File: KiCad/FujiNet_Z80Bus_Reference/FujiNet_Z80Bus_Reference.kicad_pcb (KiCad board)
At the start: 2 copper layers, 180.3 x 119.4 mm, 77 parts, among them IC1 74244N, IC10 74595N, IC11 74595N, IC12 74165N, IC13 7432N, IC14 74165N, IC15 7408N, IC16 74165N, IC17 74165N, IC19 7432N, IC2 7404N, IC20 7408N, IC21 7432N, IC22 7432N, IC3 7474N, IC4 7432N, IC5 7408N, IC6 74590N, IC7 74590N, IC8 74595N, IC9 74595N, J2 DIAG-ESP_SPI, J3 DIAG-Z80_CONTROL, J4 DIAG-ESP_CONTROL, J5 DIAG-LOCAL_ADD_HIGH, J6 DIAG-LOCAL_ADD_LOW, J7 DIAG-LOCAL_DATA, J8 DIAG-HOST_SYSTEM_BUS, Q1 2N2222 (BC337), U1 FREENOVE_ESP32-WROVER-DEV

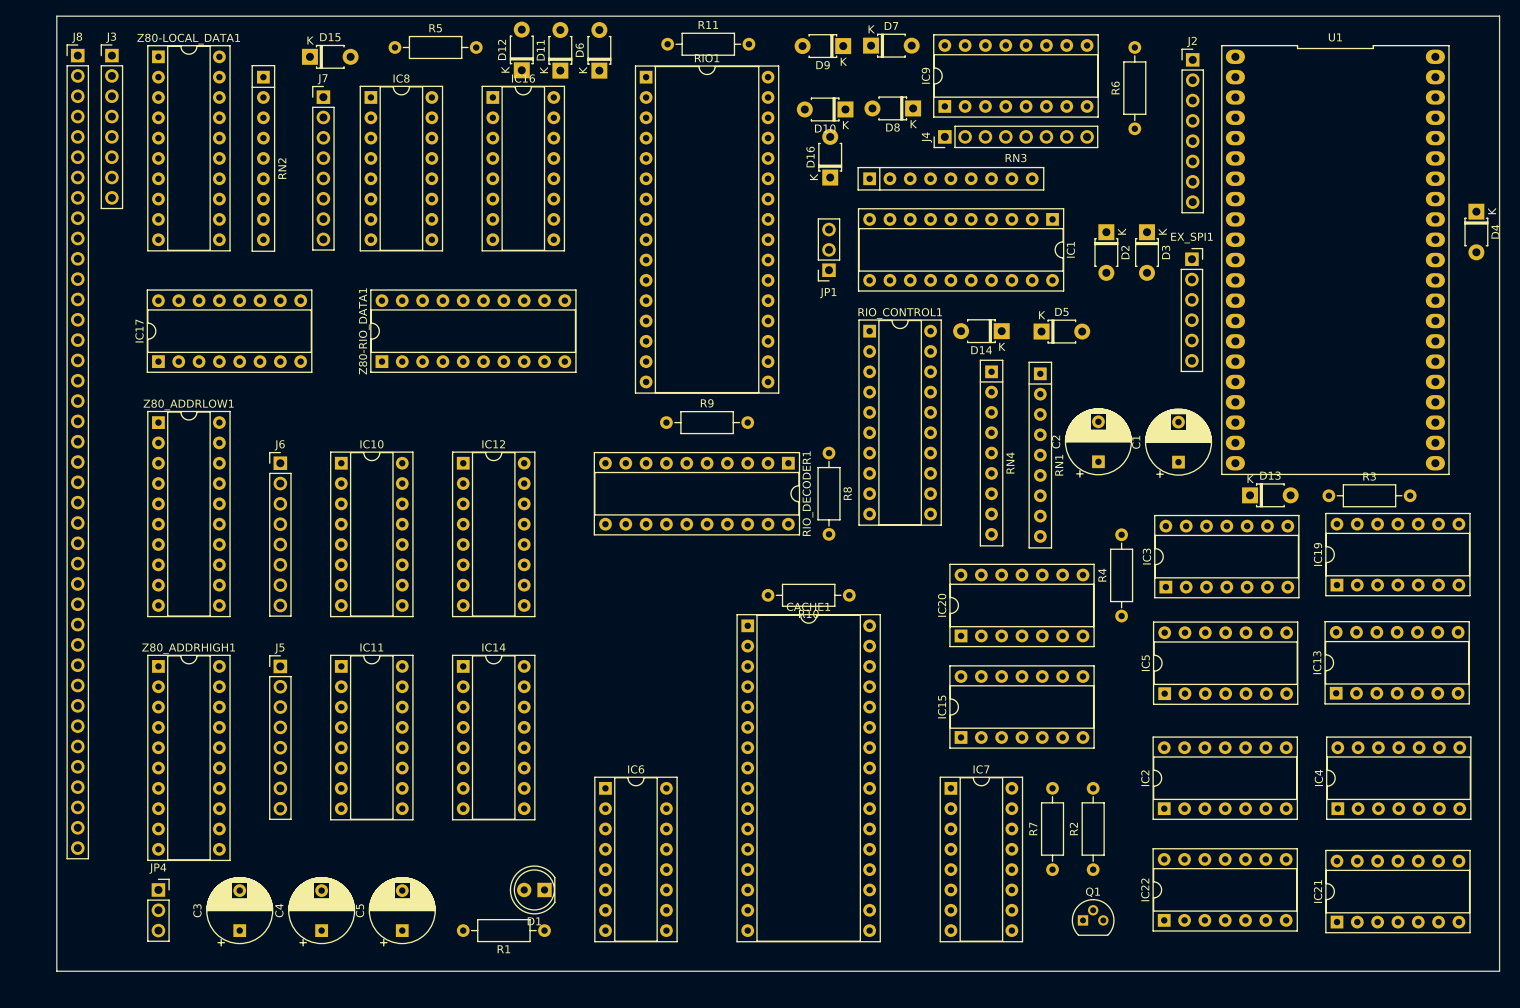
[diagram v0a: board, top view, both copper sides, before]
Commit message: Single PCB layout experiements
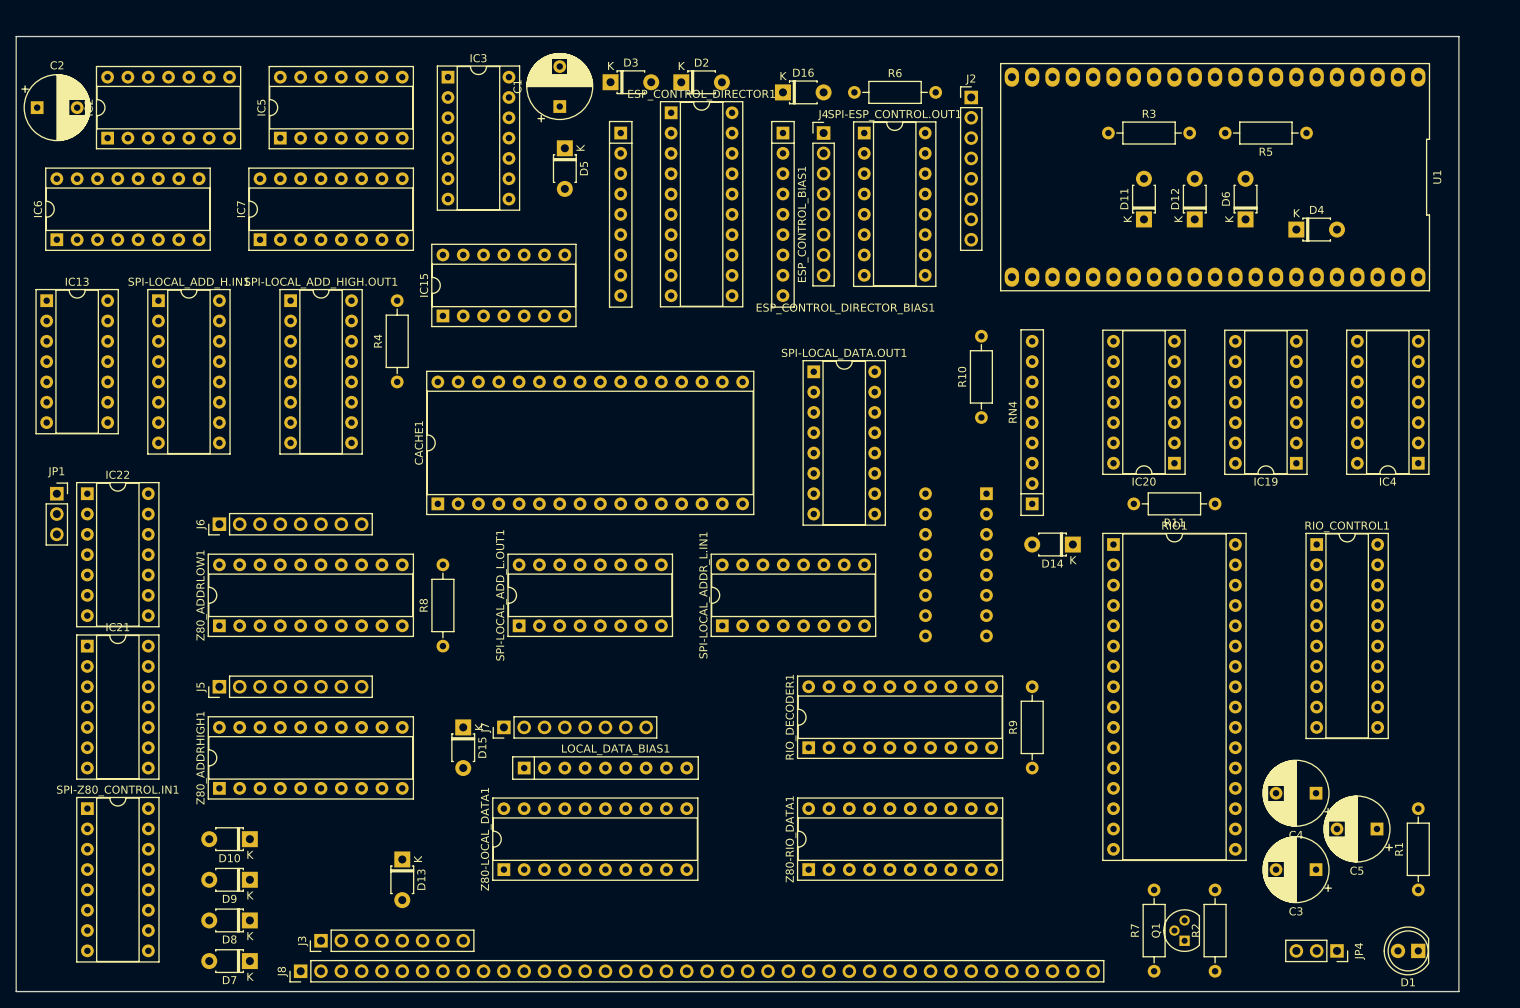
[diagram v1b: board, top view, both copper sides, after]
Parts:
- removed EX_SPI1: PINHD-1X6, Connector_PinSocket_2.54mm:PinSocket_1x06_P2.54mm_Vertical
- removed IC1: 74244N, Package_DIP:DIP-20_W7.62mm_Socket
- removed IC10, IC11, IC8, IC9: 74595N, Package_DIP:DIP-16_W7.62mm_Socket
- removed IC12, IC14, IC16, IC17: 74165N, Package_DIP:DIP-16_W7.62mm_Socket
- removed RN1, RN2, RN3: 4609M-101-103LF, Resistor_THT:R_Array_SIP9
- added ESP_CONTROL_BIAS1: 4609M-101-103LF, Resistor_THT:R_Array_SIP9, F.Cu at (133.9, 47.6)
- added ESP_CONTROL_DIRECTOR1: 74244N, Package_DIP:DIP-20_W7.62mm_Socket, F.Cu at (120.0, 45.1)
- added ESP_CONTROL_DIRECTOR_BIAS1: 4609M-101-103LF, Resistor_THT:R_Array_SIP9, F.Cu at (113.7, 47.6)
- added LOCAL_DATA_BIAS1: 4609M-101-103LF, Resistor_THT:R_Array_SIP9, F.Cu at (101.6, 127.0)
- added SPI-ESP_CONTROL.OUT1: 74595N, Package_DIP:DIP-16_W7.62mm_Socket, F.Cu at (144.1, 47.6)
- added SPI-LOCAL_ADDR_L.IN1: 74165N, Package_DIP:DIP-16_W7.62mm_Socket, F.Cu at (126.4, 109.2)
- added SPI-LOCAL_ADD_H.IN1: 74165N, Package_DIP:DIP-16_W7.62mm_Socket, F.Cu at (55.9, 68.6)
- added SPI-LOCAL_ADD_HIGH.OUT1: 74595N, Package_DIP:DIP-16_W7.62mm_Socket, F.Cu at (72.4, 68.6)
- added SPI-LOCAL_ADD_L.OUT1: 74595N, Package_DIP:DIP-16_W7.62mm_Socket, F.Cu at (101.0, 109.2)
- added SPI-LOCAL_DATA.IN1: 74165N, Package_DIP:DIP-16_W7.62mm_Socket, B.Cu at (159.4, 92.7)
- added SPI-LOCAL_DATA.OUT1: 74595N, Package_DIP:DIP-16_W7.62mm_Socket, F.Cu at (137.8, 77.5)
- added SPI-Z80_CONTROL.IN1: 74165N, Package_DIP:DIP-16_W7.62mm_Socket, F.Cu at (47.0, 132.1)
- moved IC13 168.5 mm to (41.9, 68.6), turned to 0 degrees
- moved IC21 160.0 mm to (47.0, 111.8), turned to 0 degrees
- moved IC2 156.4 mm to (49.5, 48.3)
- moved JP4 147.5 mm to (203.2, 149.9), turned to -90 degrees
- moved IC22 144.8 mm to (47.0, 92.7), turned to 0 degrees
- moved C2 139.9 mm to (40.7, 44.5), turned to 0 degrees
- moved D7 138.3 mm to (67.3, 151.1), turned to 180 degrees
- moved C3 134.8 mm to (200.6, 139.7), turned to 180 degrees
- moved D8 131.1 mm to (67.3, 146.1)
- moved IC5 130.5 mm to (71.1, 48.3)
- moved D9 127.9 mm to (67.3, 141.0)
- moved C4 125.5 mm to (200.6, 130.2), turned to 180 degrees
- moved C5 122.5 mm to (208.2, 134.6), turned to 180 degrees
- moved J8 117.8 mm to (73.7, 152.4), turned to 90 degrees
- moved D10 117.7 mm to (67.3, 135.9)
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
